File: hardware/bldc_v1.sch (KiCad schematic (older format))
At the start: 0 parts

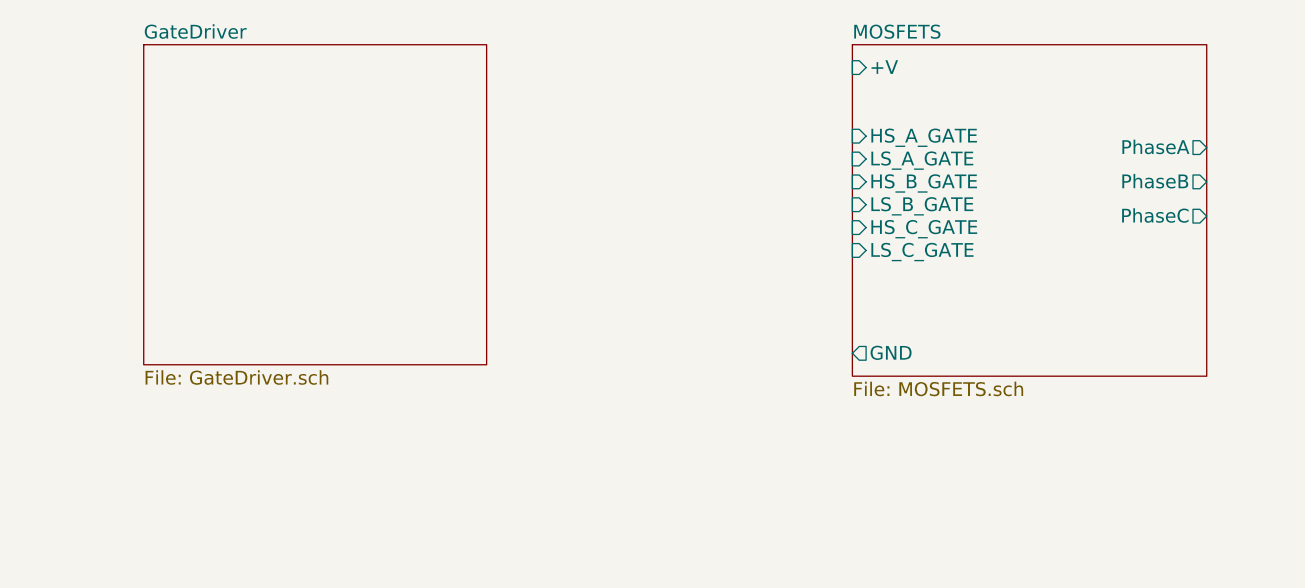
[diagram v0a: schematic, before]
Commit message: Updaated Driver section
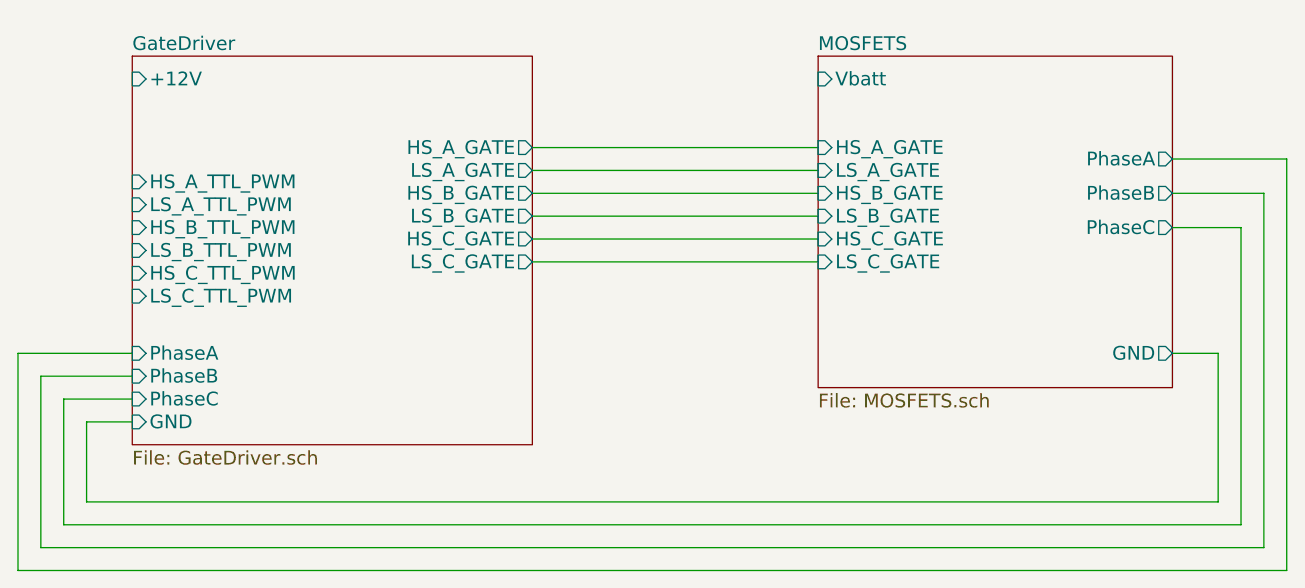
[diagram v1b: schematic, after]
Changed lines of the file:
@@
 LIBS:valves
 LIBS:infineon
+LIBS:bldc_v1-cache
 EELAYER 25 0
 EELAYER END
@@
 $EndDescr
 $Sheet
-S 1850 1450 1500 1400
+S 1800 1500 1750 1700
 U 5AAE8848
 F0 "GateDriver" 60
 F1 "GateDriver.sch" 60
+F2 "PhaseA" I L 1800 2800 60
+F3 "PhaseB" I L 1800 2900 60
+F4 "PhaseC" I L 1800 3000 60
+F5 "GND" I L 1800 3100 60
+F6 "LS_A_GATE" O R 3550 2000 60
+F7 "HS_A_GATE" O R 3550 1900 60
+F8 "LS_B_GATE" O R 3550 2200 60
+F9 "HS_B_GATE" O R 3550 2100 60
+F10 "LS_C_GATE" O R 3550 2400 60
+F11 "HS_C_GATE" O R 3550 2300 60
+F12 "LS_A_TTL_PWM" I L 1800 2150 60
+F13 "HS_A_TTL_PWM" I L 1800 2050 60
+F14 "LS_B_TTL_PWM" I L 1800 2350 60
+F15 "HS_B_TTL_PWM" I L 1800 2250 60
+F16 "LS_C_TTL_PWM" I L 1800 2550 60
+F17 "HS_C_TTL_PWM" I L 1800 2450 60
+F18 "+12V" I L 1800 1600 60
 $EndSheet
 $Sheet
-S 4950 1450 1550 1450
+S 4800 1500 1550 1450
 U 5AAE8860
 F0 "MOSFETS" 60
 F1 "MOSFETS.sch" 60
-F2 "PhaseA" O R 6500 1900 60
-F3 "+V" I L 4950 1550 60
-F4 "PhaseB" O R 6500 2050 60
-F5 "PhaseC" O R 6500 2200 60
-F6 "GND" O L 4950 2800 60
-F7 "HS_A_GATE" I L 4950 1850 60
-F8 "LS_A_GATE" I L 4950 1950 60
-F9 "HS_B_GATE" I L 4950 2050 60
-F10 "LS_B_GATE" I L 4950 2150 60
-F11 "HS_C_GATE" I L 4950 2250 60
-F12 "LS_C_GATE" I L 4950 2350 60
+F2 "PhaseA" O R 6350 1950 60
+F3 "PhaseB" O R 6350 2100 60
+F4 "PhaseC" O R 6350 2250 60
+F5 "GND" O R 6350 2800 60
+F6 "HS_A_GATE" I L 4800 1900 60
+F7 "LS_A_GATE" I L 4800 2000 60
+F8 "HS_B_GATE" I L 4800 2100 60
+F9 "LS_B_GATE" I L 4800 2200 60
+F10 "HS_C_GATE" I L 4800 2300 60
+F11 "LS_C_GATE" I L 4800 2400 60
+F12 "Vbatt" I L 4800 1600 60
 $EndSheet
+Wire Wire Line
+	3550 1900 4800 1900
+Wire Wire Line
+	3550 2000 4800 2000
+Wire Wire Line
+	3550 2100 4800 2100
+Wire Wire Line
+	3550 2200 4800 2200
+Wire Wire Line
+	3550 2300 4800 2300
+Wire Wire Line
+	3550 2400 4800 2400
+Wire Wire Line
+	6350 2800 6550 2800
+Wire Wire Line
+	6550 2800 6550 3450
+Wire Wire Line
+	6550 3450 1600 3450
+Wire Wire Line
+	1600 3450 1600 3100
+Wire Wire Line
+	1600 3100 1800 3100
+Wire Wire Line
+	6350 2250 6650 2250
+Wire Wire Line
+	6650 2250 6650 3550
+Wire Wire Line
+	6650 3550 1500 3550
+Wire Wire Line
+	1500 3550 1500 3000
+Wire Wire Line
+	1500 3000 1800 3000
+Wire Wire Line
+	6350 2100 6750 2100
+Wire Wire Line
+	6750 2100 6750 3650
+Wire Wire Line
+	6750 3650 1400 3650
+Wire Wire Line
+	1400 3650 1400 2900
+Wire Wire Line
+	1400 2900 1800 2900
+Wire Wire Line
+	6350 1950 6850 1950
+Wire Wire Line
+	6850 1950 6850 3750
+Wire Wire Line
+	6850 3750 1300 3750
+Wire Wire Line
+	1300 3750 1300 2800
+Wire Wire Line
+	1300 2800 1800 2800
 $EndSCHEMATC
